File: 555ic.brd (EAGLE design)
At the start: 19.1 x 31.8 mm, 5 parts, among them IC1 LM555N

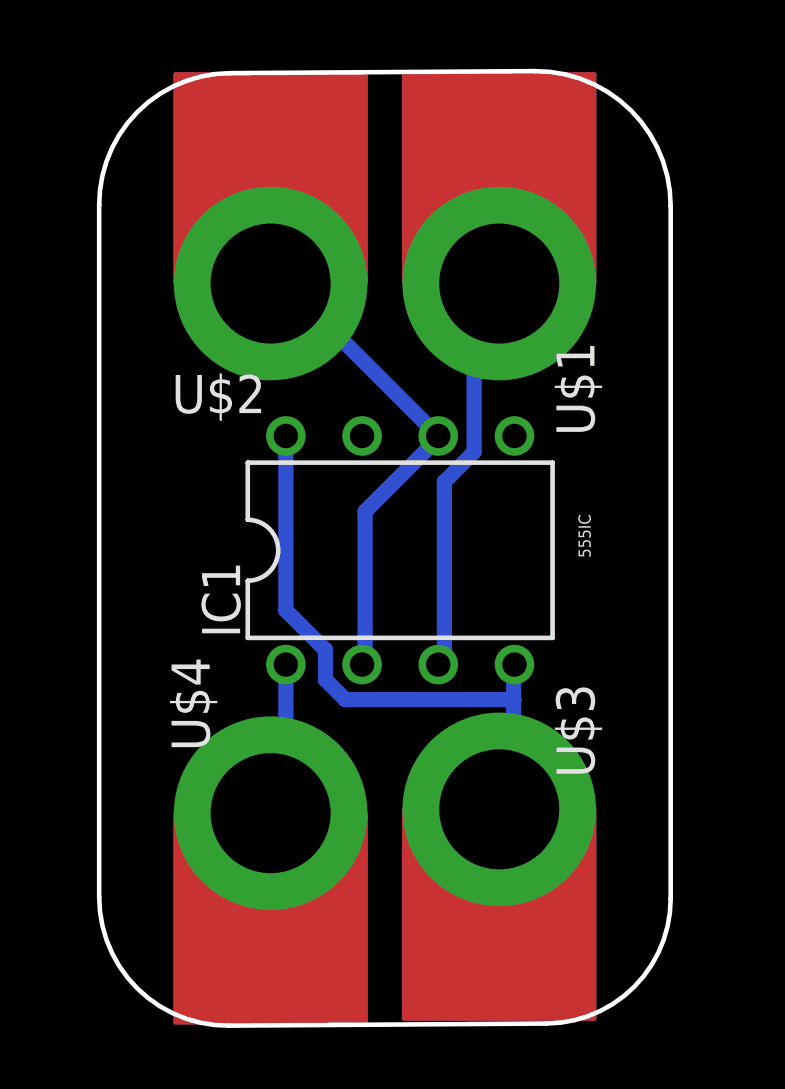
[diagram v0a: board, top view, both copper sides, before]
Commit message: Updated 555ic.b#1
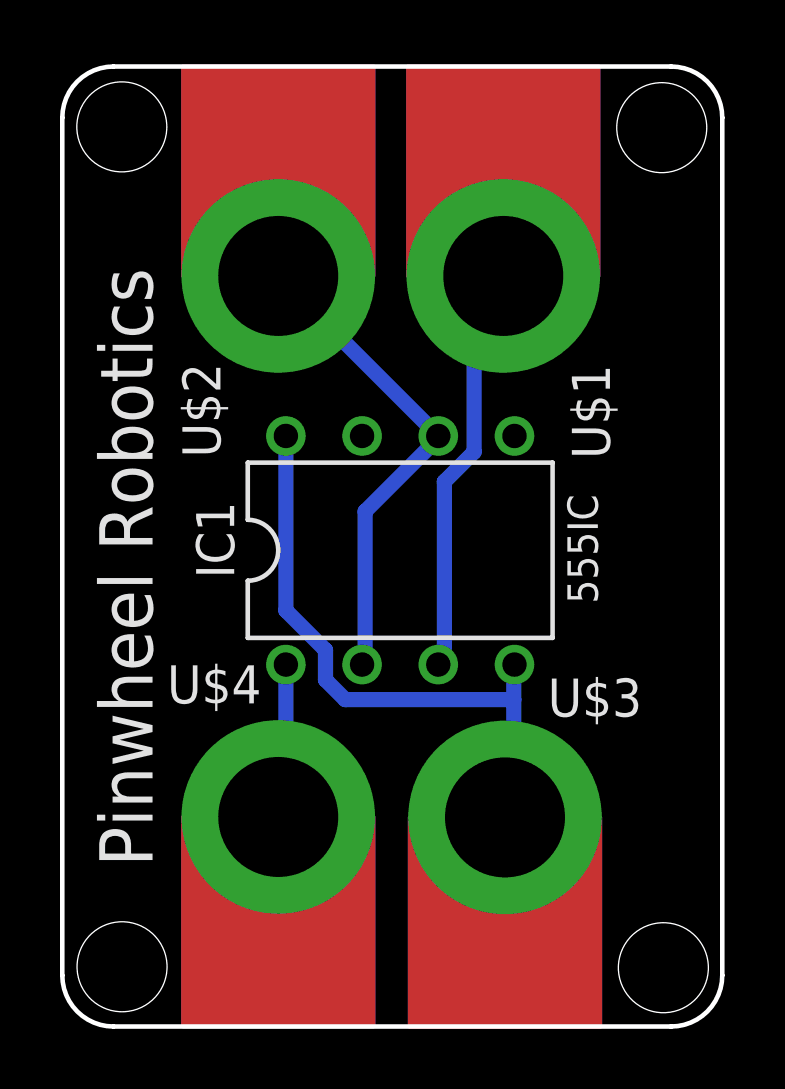
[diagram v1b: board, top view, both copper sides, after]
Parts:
- moved U$2 0.36 mm to (4.70, 25.0)
- moved U$3 0.33 mm to (12.3, 6.97)
- moved U$1 0.29 mm to (12.2, 25.0)
- moved U$4 0.28 mm to (4.70, 6.99)
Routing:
- net GND: track 5.17 -> 5.77 mm
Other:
- board size 19.1 x 31.8 mm -> 22 x 32 mm
- board text added: "Pinwheel Robotics"
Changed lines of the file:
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@@
 <setting verticaltext="up"/>
 </settings>
-<grid distance="50" unitdist="mil" unit="mm" style="lines" multiple="1" display="yes" altdistance="5" altunitdist="mil" altunit="mm"/>
+<grid distance="0.5" unitdist="mm" unit="mm" style="lines" multiple="1" display="yes" altdistance="5" altunitdist="mil" altunit="mm"/>
 <layers>
 <layer number="1" name="Top" color="4" fill="1" visible="yes" active="yes"/>
@@
 <layer number="43" name="vRestrict" color="2" fill="10" visible="yes" active="yes"/>
 <layer number="44" name="Drills" color="7" fill="1" visible="no" active="yes"/>
-<layer number="45" name="Holes" color="7" fill="1" visible="no" active="yes"/>
+<layer number="45" name="Holes" color="7" fill="1" visible="yes" active="yes"/>
 <layer number="46" name="Milling" color="3" fill="1" visible="no" active="yes"/>
 <layer number="47" name="Measures" color="7" fill="1" visible="no" active="yes"/>
@@
 <board>
 <plain>
-<wire x1="13.642678125" y1="0.09941875" x2="3.04553125" y2="0.028771875" width="0.1524" layer="20"/>
-<wire x1="3.04553125" y1="0.028771875" x2="-1.27" y2="4.315628125" width="0.1524" layer="20" curve="-90.384308"/>
-<wire x1="-1.27" y1="4.315628125" x2="-1.27" y2="27.393453125" width="0.1524" layer="20"/>
-<wire x1="-1.27" y1="27.393453125" x2="3.08645" y2="31.77904375" width="0.1524" layer="20" curve="-89.618031"/>
-<wire x1="3.08645" y1="31.77904375" x2="13.249803125" y2="31.8468" width="0.1524" layer="20"/>
-<wire x1="13.249803125" y1="31.8468" x2="17.78" y2="27.346703125" width="0.1524" layer="20" curve="-90.382759"/>
-<wire x1="17.78" y1="27.346703125" x2="17.78" y2="4.2644125" width="0.1524" layer="20"/>
-<wire x1="17.78" y1="4.2644125" x2="13.642678125" y2="0.09941875" width="0.1524" layer="20" curve="-89.618048"/>
-<text x="15.113" y="15.621" size="0.4064" layer="21" rot="R90">555IC</text>
+<text x="15.353" y="14.099" size="1.016" layer="21" rot="R90">555IC</text>
+<hole x="-0.516" y="29.988" drill="3"/>
+<hole x="17.482" y="29.962" drill="3"/>
+<hole x="17.536" y="1.96" drill="3"/>
+<hole x="-0.508" y="1.992" drill="3"/>
+<wire x1="19.5" y1="30.292896875" x2="19.5" y2="1.707103125" width="0.1524" layer="20"/>
+<wire x1="19.5" y1="1.707103125" x2="17.792896875" y2="0" width="0.1524" layer="20" curve="-90"/>
+<wire x1="17.792896875" y1="0" x2="-0.792896875" y2="0" width="0.1524" layer="20"/>
+<wire x1="-0.792896875" y1="0" x2="-2.5" y2="1.707103125" width="0.1524" layer="20" curve="-90"/>
+<wire x1="-2.5" y1="1.707103125" x2="-2.5" y2="30.292896875" width="0.1524" layer="20"/>
+<wire x1="-2.5" y1="30.292896875" x2="-0.792896875" y2="32" width="0.1524" layer="20" curve="-90"/>
+<wire x1="-0.792896875" y1="32" x2="17.792896875" y2="32" width="0.1524" layer="20"/>
+<wire x1="17.792896875" y1="32" x2="19.5" y2="30.292896875" width="0.1524" layer="20" curve="-90"/>
+<text x="0.508" y="5.334" size="1.778" layer="21" rot="R90">Pinwheel Robotics</text>
 </plain>
 <attributes>
@@
 <elements>
 <element name="IC1" library="linear" library_urn="urn:adsk.eagle:library:262" package="DIL08" package3d_urn="urn:adsk.eagle:package:16409/2" value="LM555N" x="8.763" y="15.875" smashed="yes">
-<attribute name="NAME" x="3.429" y="12.954" size="1.27" layer="25" ratio="10" rot="R90"/>
+<attribute name="NAME" x="3.231" y="14.94" size="1.27" layer="25" ratio="10" rot="R90"/>
 <attribute name="POPULARITY" value="0" x="27.813" y="-20.955" size="1.778" layer="27" display="off"/>
 <attribute name="VALUE" x="5.207" y="15.24" size="1.27" layer="27" ratio="10"/>
 </element>
-<element name="U$1" library="microbit" package="MICROBIT_PAD" value="MICROBIT_PAD" x="12.065" y="24.765" smashed="yes" rot="R180">
-<attribute name="NAME" x="15.24" y="19.685" size="1.27" layer="21" rot="R90"/>
+<element name="U$1" library="microbit" package="MICROBIT_PAD" value="MICROBIT_PAD" x="12.2" y="25.019" smashed="yes" rot="R180">
+<attribute name="NAME" x="15.756" y="18.923" size="1.27" layer="21" rot="R90"/>
 </element>
-<element name="U$2" library="microbit" package="MICROBIT_PAD" value="MICROBIT_PAD" x="4.445" y="24.765" smashed="yes" rot="R180">
-<attribute name="NAME" x="1.143" y="20.447" size="1.27" layer="21"/>
+<element name="U$2" library="microbit" package="MICROBIT_PAD" value="MICROBIT_PAD" x="4.699" y="25.019" smashed="yes" rot="R180">
+<attribute name="NAME" x="2.773" y="18.971" size="1.27" layer="21" rot="R90"/>
 </element>
-<element name="U$3" library="microbit" package="MICROBIT_PAD" value="MICROBIT_PAD" x="12.065" y="7.239" smashed="yes">
-<attribute name="NAME" x="13.97" y="11.43" size="1.27" layer="21" rot="R270"/>
+<element name="U$3" library="microbit" package="MICROBIT_PAD" value="MICROBIT_PAD" x="12.257" y="6.97" smashed="yes">
+<attribute name="NAME" x="13.682" y="10.33" size="1.27" layer="21"/>
 </element>
-<element name="U$4" library="microbit" package="MICROBIT_PAD" value="MICROBIT_PAD" x="4.445" y="7.112" smashed="yes">
-<attribute name="NAME" x="1.143" y="12.319" size="1.27" layer="21" rot="R270"/>
+<element name="U$4" library="microbit" package="MICROBIT_PAD" value="MICROBIT_PAD" x="4.699" y="6.985" smashed="yes">
+<attribute name="NAME" x="4.137" y="12.041" size="1.27" layer="21" rot="R180"/>
 </element>
 </elements>
@@
 <contactref element="IC1" pad="4"/>
 <contactref element="U$3" pad="PAD"/>
-<wire x1="12.5476" y1="7.5946" x2="12.5476" y2="10.8966" width="0.508" layer="16"/>
+<wire x1="12.5476" y1="7.018434375" x2="12.5476" y2="10.8966" width="0.508" layer="16"/>
 <wire x1="12.5476" y1="10.8966" x2="12.5476" y2="11.8872" width="0.508" layer="16"/>
-<wire x1="12.2174" y1="7.2644" x2="12.5476" y2="7.5946" width="0.508" layer="16"/>
 <wire x1="12.5476" y1="11.8872" x2="12.573" y2="12.065" width="0.508" layer="16"/>
-<wire x1="12.2174" y1="7.2644" x2="12.065" y2="7.239" width="0.508" layer="16"/>
+<wire x1="12.5476" y1="7.018434375" x2="12.257" y2="6.97" width="0.508" layer="16"/>
 <wire x1="4.953" y1="13.8684" x2="4.953" y2="19.685" width="0.508" layer="16"/>
 <wire x1="6.2738" y1="12.5476" x2="4.953" y2="13.8684" width="0.508" layer="16"/>
@@
 <wire x1="11.2268" y1="19.1516" x2="10.2362" y2="18.161" width="0.508" layer="16"/>
 <wire x1="11.2268" y1="24.1046" x2="11.2268" y2="19.1516" width="0.508" layer="16"/>
-<wire x1="11.8872" y1="24.765" x2="11.2268" y2="24.1046" width="0.508" layer="16"/>
+<wire x1="12.1412" y1="25.019" x2="11.2268" y2="24.1046" width="0.508" layer="16"/>
 <wire x1="10.2362" y1="12.2174" x2="10.033" y2="12.065" width="0.508" layer="16"/>
-<wire x1="11.8872" y1="24.765" x2="12.065" y2="24.765" width="0.508" layer="16"/>
+<wire x1="12.1412" y1="25.019" x2="12.2" y2="25.019" width="0.508" layer="16"/>
 </signal>
 <signal name="N$2">
@@
 <wire x1="7.5946" y1="12.2174" x2="7.493" y2="12.065" width="0.508" layer="16"/>
 <wire x1="9.906" y1="19.4818" x2="10.033" y2="19.685" width="0.508" layer="16"/>
-<wire x1="4.953" y1="24.765" x2="10.033" y2="19.685" width="0.508" layer="16"/>
-<wire x1="4.445" y1="24.765" x2="4.953" y2="24.765" width="0.508" layer="16"/>
+<wire x1="4.699" y1="25.019" x2="10.033" y2="19.685" width="0.508" layer="16"/>
 </signal>
 <signal name="GND">
 <contactref element="IC1" pad="1"/>
 <contactref element="U$4" pad="PAD"/>
-<wire x1="4.953" y1="7.5946" x2="4.953" y2="12.065" width="0.508" layer="16"/>
-<wire x1="4.6228" y1="7.2644" x2="4.953" y2="7.5946" width="0.508" layer="16"/>
-<wire x1="4.6228" y1="7.2644" x2="4.445" y2="7.112" width="0.508" layer="16"/>
+<wire x1="4.953" y1="12.065" x2="4.953" y2="6.688665625" width="0.508" layer="16"/>
+<wire x1="4.953" y1="6.688665625" x2="4.699" y2="6.985" width="0.508" layer="16"/>
 </signal>
 </signals>

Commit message: New Updates
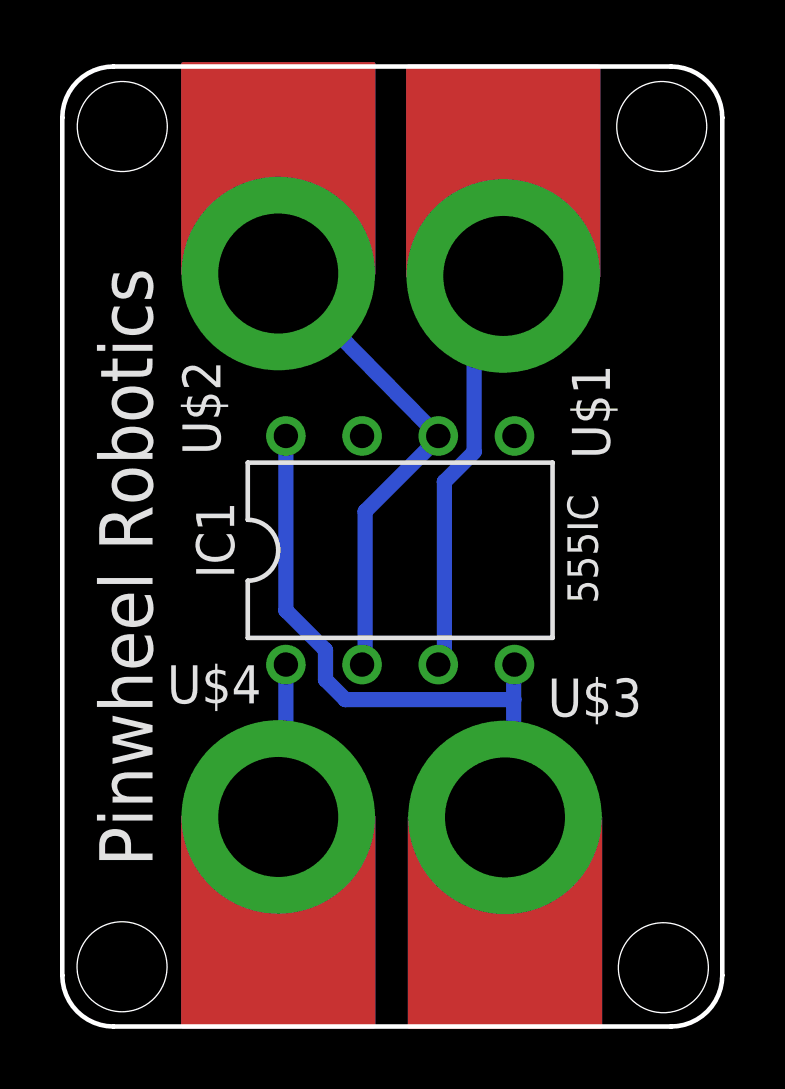
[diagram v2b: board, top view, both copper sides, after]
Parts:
- moved U$2 0.08 mm to (4.70, 25.1)
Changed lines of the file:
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@@
 <drawing>
 <settings>
-<setting alwaysvectorfont="yes"/>
+<setting alwaysvectorfont="no"/>
 <setting verticaltext="up"/>
 </settings>
@@
 <plain>
 <text x="15.353" y="14.099" size="1.016" layer="21" rot="R90">555IC</text>
-<hole x="-0.516" y="29.988" drill="3"/>
-<hole x="17.482" y="29.962" drill="3"/>
+<hole x="-0.5" y="30" drill="3"/>
+<hole x="17.482" y="30" drill="3"/>
 <hole x="17.536" y="1.96" drill="3"/>
 <hole x="-0.508" y="1.992" drill="3"/>
@@
 <attribute name="NAME" x="15.756" y="18.923" size="1.27" layer="21" rot="R90"/>
 </element>
-<element name="U$2" library="microbit" package="MICROBIT_PAD" value="MICROBIT_PAD" x="4.699" y="25.019" smashed="yes" rot="R180">
-<attribute name="NAME" x="2.773" y="18.971" size="1.27" layer="21" rot="R90"/>
+<element name="U$2" library="microbit" package="MICROBIT_PAD" value="MICROBIT_PAD" x="4.699" y="25.1" smashed="yes" rot="R180">
+<attribute name="NAME" x="2.773" y="19.052" size="1.27" layer="21" rot="R90"/>
 </element>
 <element name="U$3" library="microbit" package="MICROBIT_PAD" value="MICROBIT_PAD" x="12.257" y="6.97" smashed="yes">
@@
 <wire x1="7.5946" y1="12.2174" x2="7.493" y2="12.065" width="0.508" layer="16"/>
 <wire x1="9.906" y1="19.4818" x2="10.033" y2="19.685" width="0.508" layer="16"/>
-<wire x1="4.699" y1="25.019" x2="10.033" y2="19.685" width="0.508" layer="16"/>
+<wire x1="4.699" y1="25.1" x2="10.033" y2="19.685" width="0.508" layer="16"/>
 </signal>
 <signal name="GND">

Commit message: New Update
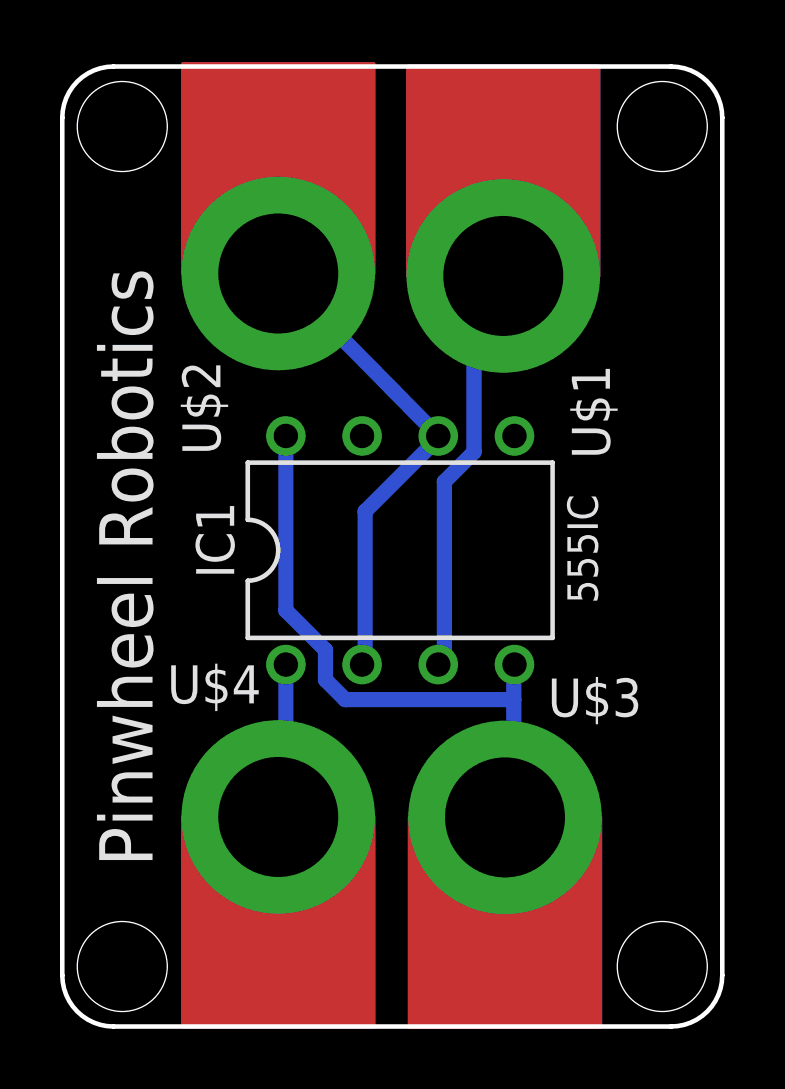
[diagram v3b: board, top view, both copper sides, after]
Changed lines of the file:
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@@
 <text x="15.353" y="14.099" size="1.016" layer="21" rot="R90">555IC</text>
 <hole x="-0.5" y="30" drill="3"/>
-<hole x="17.482" y="30" drill="3"/>
-<hole x="17.536" y="1.96" drill="3"/>
-<hole x="-0.508" y="1.992" drill="3"/>
+<hole x="17.5" y="30" drill="3"/>
+<hole x="17.5" y="2" drill="3"/>
+<hole x="-0.5" y="2" drill="3"/>
 <wire x1="19.5" y1="30.292896875" x2="19.5" y2="1.707103125" width="0.1524" layer="20"/>
 <wire x1="19.5" y1="1.707103125" x2="17.792896875" y2="0" width="0.1524" layer="20" curve="-90"/>
